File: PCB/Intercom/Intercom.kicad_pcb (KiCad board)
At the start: 4 copper layers, 49.3 x 39.8 mm, 33 parts, among them J1 Reset, J2 Battery, J3 TC2030-USB-NL-DS, J5 USB-C-Socket-H, Q1 CJ2301, SW2 SW_Push, U2 MAX98357A, U3 TP4054, U4 ME6211C33M5G-N, U5 L, U6 ESP32-S3-MINI-1, U7 R

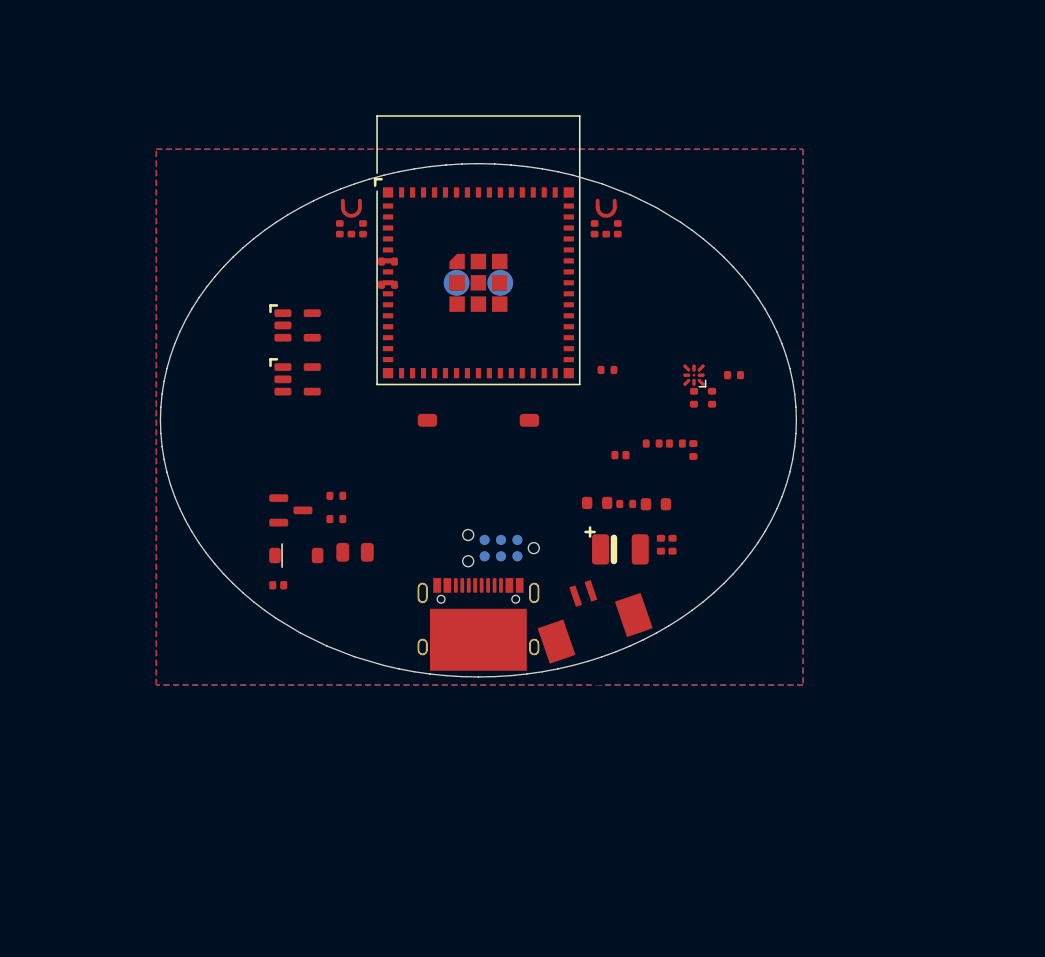
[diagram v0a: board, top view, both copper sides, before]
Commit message: Started new Intercom
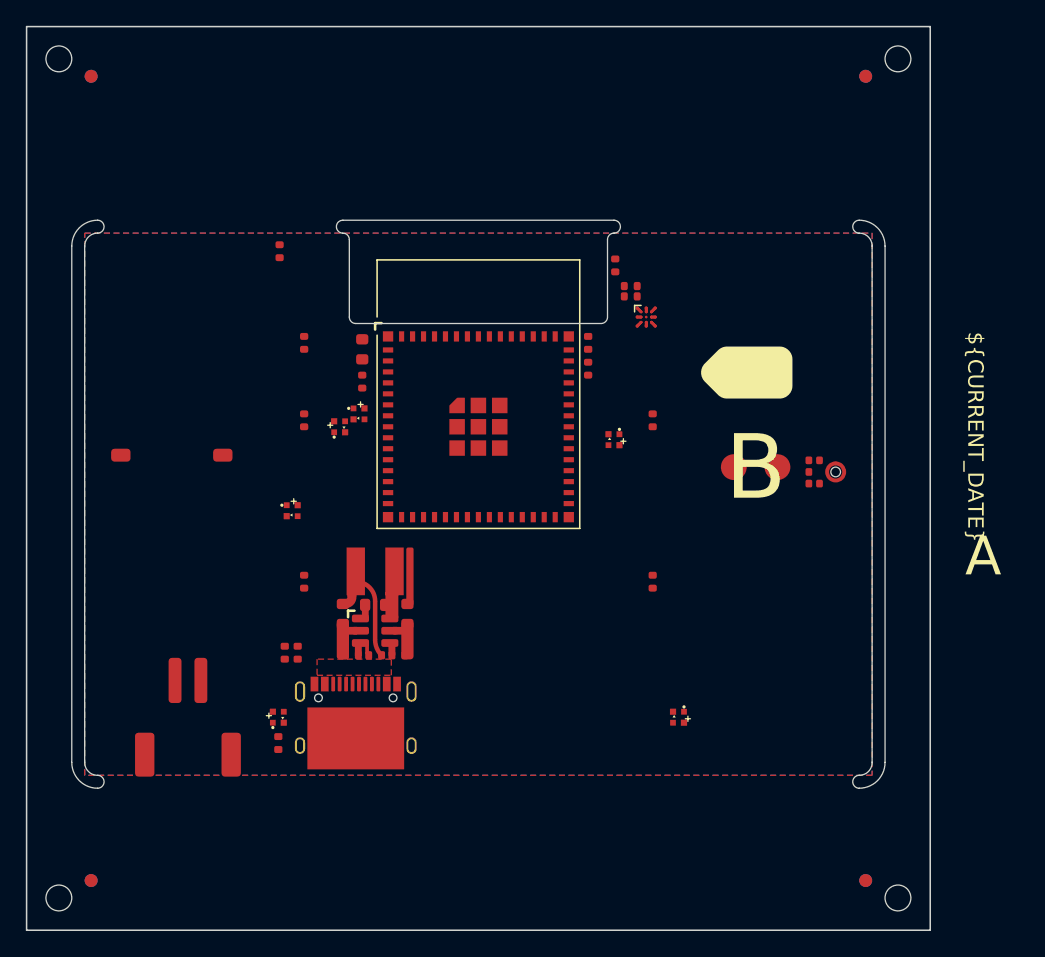
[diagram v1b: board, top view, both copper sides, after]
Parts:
- removed C13: 10uF, RevK:C_0402
- removed J3: TC2030-USB-NL-DS, RevK:Tag-Connect_TC2030-IDC-NL_2x03_P1.27mm_Vertical
- removed Q1: CJ2301, RevK:SOT-23
- removed R5: 5K1, RevK:R_0402
- removed SW2: SW_Push, RevK:TS-1092S-B3D2-G
- removed U3: TP4054, RevK:SOT-23-5
- removed U5: L, RevK:ICS43434_MEMS_Mic_Open
- removed U7: R, RevK:ICS43434_MEMS_Mic_Open
- added C11: 100nF, RevK:C_0402, F.Cu at (86.5, 89.5)
- added C12: 10uF, RevK:C_0402, F.Cu at (111.8, 85.1)
- added C15: 100nF, RevK:C_0402, F.Cu at (91.0, 92.5)
- added C16: 22uF, RevK:C_0603, F.Cu at (91.0, 90.0)
- added D4: XL-1010RGBC-WS2812B, RevK:SMD1010, F.Cu at (89.2, 96.0)
- added D5: XL-1010RGBC-WS2812B, RevK:SMD1010, F.Cu at (110.5, 97.0)
- added D6: XL-1010RGBC-WS2812B, RevK:SMD1010, F.Cu at (85.6, 102.5)
- added J4: TC2030-USB-NL-DS, RevK:Tag-Connect_TC2030-IDC-NL_2x03_P1.27mm_Vertical, F.Cu at (120.8, 91.8)
- added L1: 10uH, RevK:L_4x4_, F.Cu at (92.0, 107.2)
- added PCB1: 70x70, RevK:PCB7070, F.Cu at (100.0, 100.0)
- added R4: 10K, RevK:R_0402, F.Cu at (84.5, 120.5)
- added R7: 5K1, RevK:R_0402, F.Cu at (86.0, 113.5)
- added SW1: SW_Push, RevK:TS-1092S-B3D2-G, F.Cu at (76.2, 98.2)
- added U1: MD8942, RevK:SOT-23-6-MD8942, F.Cu at (92.0, 111.8)
- added V2: ~, RevK:VCUT70N, F.Cu at (100.0, 123.0)
- added V3: ~, RevK:VCUT70N, F.Cu at (100.0, 81.0)
- C1: value 220uF Tant -> 10uF 35V; footprint RevK:CP_EIA-3528-21_Kemet-B -> RevK:C_0603_
- C2: value 100nF -> 10uF 6.3V; footprint RevK:C_0402 -> RevK:C_0603_
- C3: value 22uF -> 100nF; footprint RevK:C_0603 -> RevK:C_0603_
- C4: value 100uF -> 1uF; footprint RevK:C_0805 -> RevK:C_0402
- C5: value 10uF 35V -> 100nF; footprint RevK:C_0603 -> RevK:C_0402
- C7, C8: value 10uF -> 100nF
- C9: value 1uF -> 100nF
- D1, D3: value ~ -> XL-1010RGBC-WS2812B; footprint RevK:DFN1006-2L -> RevK:SMD1010
- D2: value MBR0530 -> XL-1010RGBC-WS2812B; footprint RevK:D_SOD-123 -> RevK:SMD1010
- J1: moved to F.Cu
- J2: value Battery -> JST-PH-SM4-TB; footprint RevK:1.25T-2PWT (Molex 532610271) -> RevK:JST_PH_S2B-PH-SM4-TB_1x02-1MP_P2.00mm_Horizontal
- R1: value 10K -> 124k; footprint RevK:R_0402 -> RevK:R_0402_
- R2: value 10K -> 39k2; footprint RevK:R_0402 -> RevK:R_0402_
- R3: value 10K -> 1M; footprint RevK:R_0402 -> RevK:R_0402_
- R6: value 5K1 -> 10K
- R8: value 634K -> 5K1
- U2: value MAX98357A -> ESP32-S3-MINI-1; footprint RevK:WLP-1.437mmx1.347mm-0.21mm-ball -> RevK:ESP32-S3-MINI-1
- U4: value ME6211C33M5G-N -> R; footprint RevK:SOT-23-5 -> RevK:ICS43434_MEMS_Mic
- U6: value ESP32-S3-MINI-1 -> MAX98357A; footprint RevK:ESP32-S3-MINI-1 -> RevK:WLP-1.437mmx1.347mm-0.21mm-ball
- moved U4 41.5 mm to (126.9, 99.5)
- moved R8 40.9 mm to (85.0, 113.5), turned to -90 degrees
- moved C9 32.5 mm to (84.6, 82.4), turned to -90 degrees
- moved D2 32.1 mm to (115.5, 118.5), turned to -90 degrees
- moved J2 32.1 mm to (77.5, 118.5), turned to 0 degrees
- moved C7 31.8 mm to (86.5, 108.0), turned to 90 degrees
- moved R2 30.0 mm to (90.2, 113.7)
- moved C5 28.0 mm to (86.5, 95.5), turned to 90 degrees
- moved J1 25.8 mm to (121.5, 99.1), turned to 0 degrees
- moved C6 23.9 mm to (113.5, 95.5), turned to -90 degrees
- moved C2 23.5 mm to (89.5, 110.5), turned to -90 degrees
- moved C4 22.9 mm to (108.5, 91.5), turned to -90 degrees
- moved D3 20.5 mm to (90.8, 95.0)
- moved C3 18.9 mm to (92.0, 109.8)
- moved C10 17.7 mm to (110.6, 83.5), turned to -90 degrees
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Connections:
- C14 pad 1: +3V3 -> +5V
- C4 pad 1: +3V3 -> Net-(U2-EN)
- C5 pad 1: DC -> GND
- C5 pad 2: GND -> +5V
- C6 pad 2: +3V3 -> +5V
- C7 pad 1: +3V3 -> GND
- C7 pad 2: GND -> +5V
- C8 pad 1: +3V3 -> GND
- C8 pad 2: GND -> +5V
- C9 pad 1: Net-(U6-EN) -> GND
- C9 pad 2: GND -> +5V
- D1 pad 1: GND -> Net-(D1-O)
- D1 pad 2: VBAT -> +5V
- D2 pad 1: Net-(D2-K) -> Net-(D2-O)
- D2 pad 2: VBUS -> +5V
- D3 pad 1: GND -> Net-(D1-I)
- D3 pad 2: PUSH -> +5V
- J2 pad 1: VBAT -> Net-(J2-Pin_1)
- J2 pad 2: GND -> Net-(J2-Pin_2)
- J5 pad A4: DC -> +5V
- J5 pad A9: DC -> +5V
- J5 pad B4: DC -> +5V
- J5 pad B9: DC -> +5V
- R6 pad 1: GND -> +3V3
- R6 pad 2: Net-(J5-CC2) -> Net-(U2-EN)
- R8 pad 1: Net-(U2-~{SD_MODE}) -> GND
- R8 pad 2: SKPPWR -> Net-(J5-CC2)
- U4 pad 1: Net-(D2-K) -> MICWS
- U4 pad 2: GND -> +3V3
- U4 pad 3: Net-(D2-K) -> GND
- U4 pad 4: unconnected-(U4-NC-Pad4) -> MICSCK
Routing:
- added copper zone on F.Cu, net +5V
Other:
- board size 49.3 x 39.8 mm -> 70 x 70 mm
- copper layers 4 -> 2
- board text added: "${CURRENT_DATE}"
- board text added: "A"
